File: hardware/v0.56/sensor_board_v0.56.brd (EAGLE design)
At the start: 50.8 x 50.8 mm, 73 parts, among them J3 USB-MICROB, U1 TPS61090RSAR, U10 TSL2591, U11 915MHz, U3 OPA344, U4 SI7021, U5 ATMEGA328P-MU, U6 ADMP401, U7 PMS7003, U8 MCP1703CB, U9 BMP280, X1 16 MHz

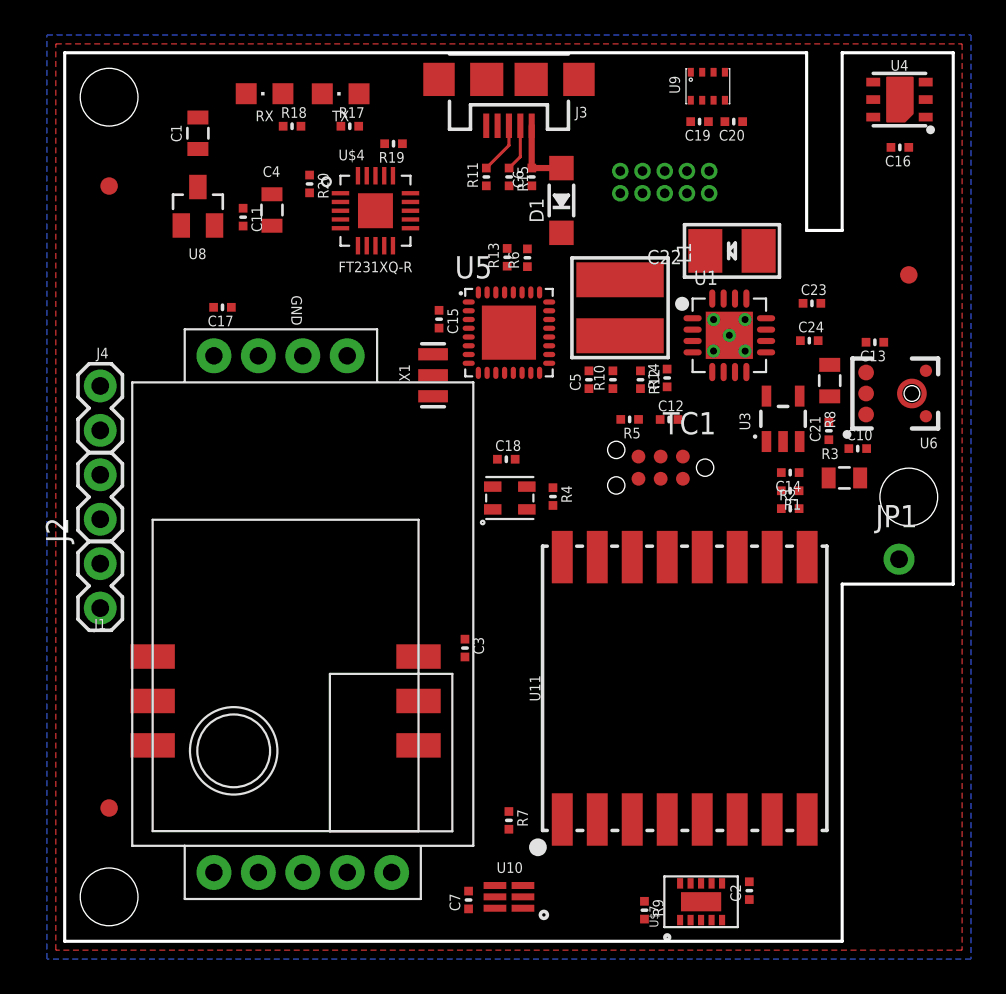
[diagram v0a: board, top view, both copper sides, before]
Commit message: Adjustments
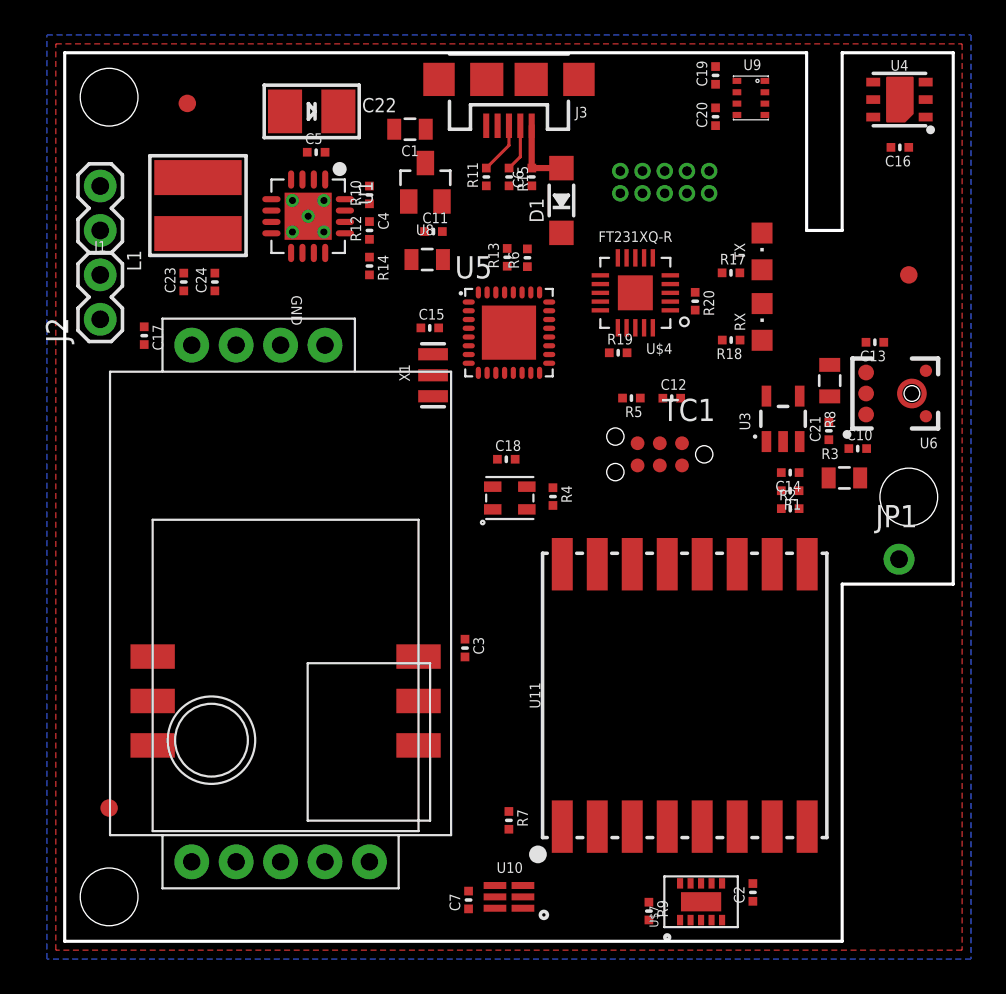
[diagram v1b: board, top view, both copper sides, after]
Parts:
- removed J4: (no value), SparkFun-Connectors:1X02
- moved C23 35.9 mm to (6.81, 37.7), turned to 90 degrees
- moved C24 34.2 mm to (8.59, 37.7), turned to 90 degrees
- moved RX 31.3 mm to (39.9, 35.4), turned to 0 degrees
- moved R18 27.9 mm to (38.1, 34.4), turned to 180 degrees
- moved TX 25.7 mm to (39.9, 39.4), turned to 0 degrees
- moved C22 25.3 mm to (14.1, 47.4), turned to 0 degrees
- moved U1 25.0 mm to (13.9, 41.5), turned to 270 degrees
- moved L1 24.8 mm to (7.62, 42.1), turned to 90 degrees
- moved R17 23.3 mm to (38.1, 38.2)
- moved R20 23.0 mm to (36.0, 36.6)
- moved J1 21.6 mm to (2.03, 40.6)
- moved C5 20.3 mm to (14.4, 45.1), turned to 0 degrees
- moved R14 18.2 mm to (17.4, 38.6), turned to 270 degrees
- moved R12 17.7 mm to (17.4, 40.6), turned to 90 degrees
- moved R19 17.5 mm to (31.6, 33.6), turned to 0 degrees
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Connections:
- removed net 5.0V: C22.+, C5.2, R10.2, U1.1, U1.15, U1.16
- new net 5V: C17.2, C22.+, C5.2, R10.2, U$6.VIN, U1.1, U1.15, U1.16
- net GND: now also U1.9; no longer J4.1
- net PWR: no longer C17.2, U$6.VIN
- net VCC: no longer J4.2
